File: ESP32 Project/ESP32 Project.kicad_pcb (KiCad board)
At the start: 4 copper layers, 49 x 38.3 mm, 27 parts, among them P1 USB_C_Plug_USB2.0, U1 ESP32-S3-WROOM-1-N8R2, U2 AMS1117, U3 BMP390, U4 INA219AxD, U5 LM75B, U6 SHTC3

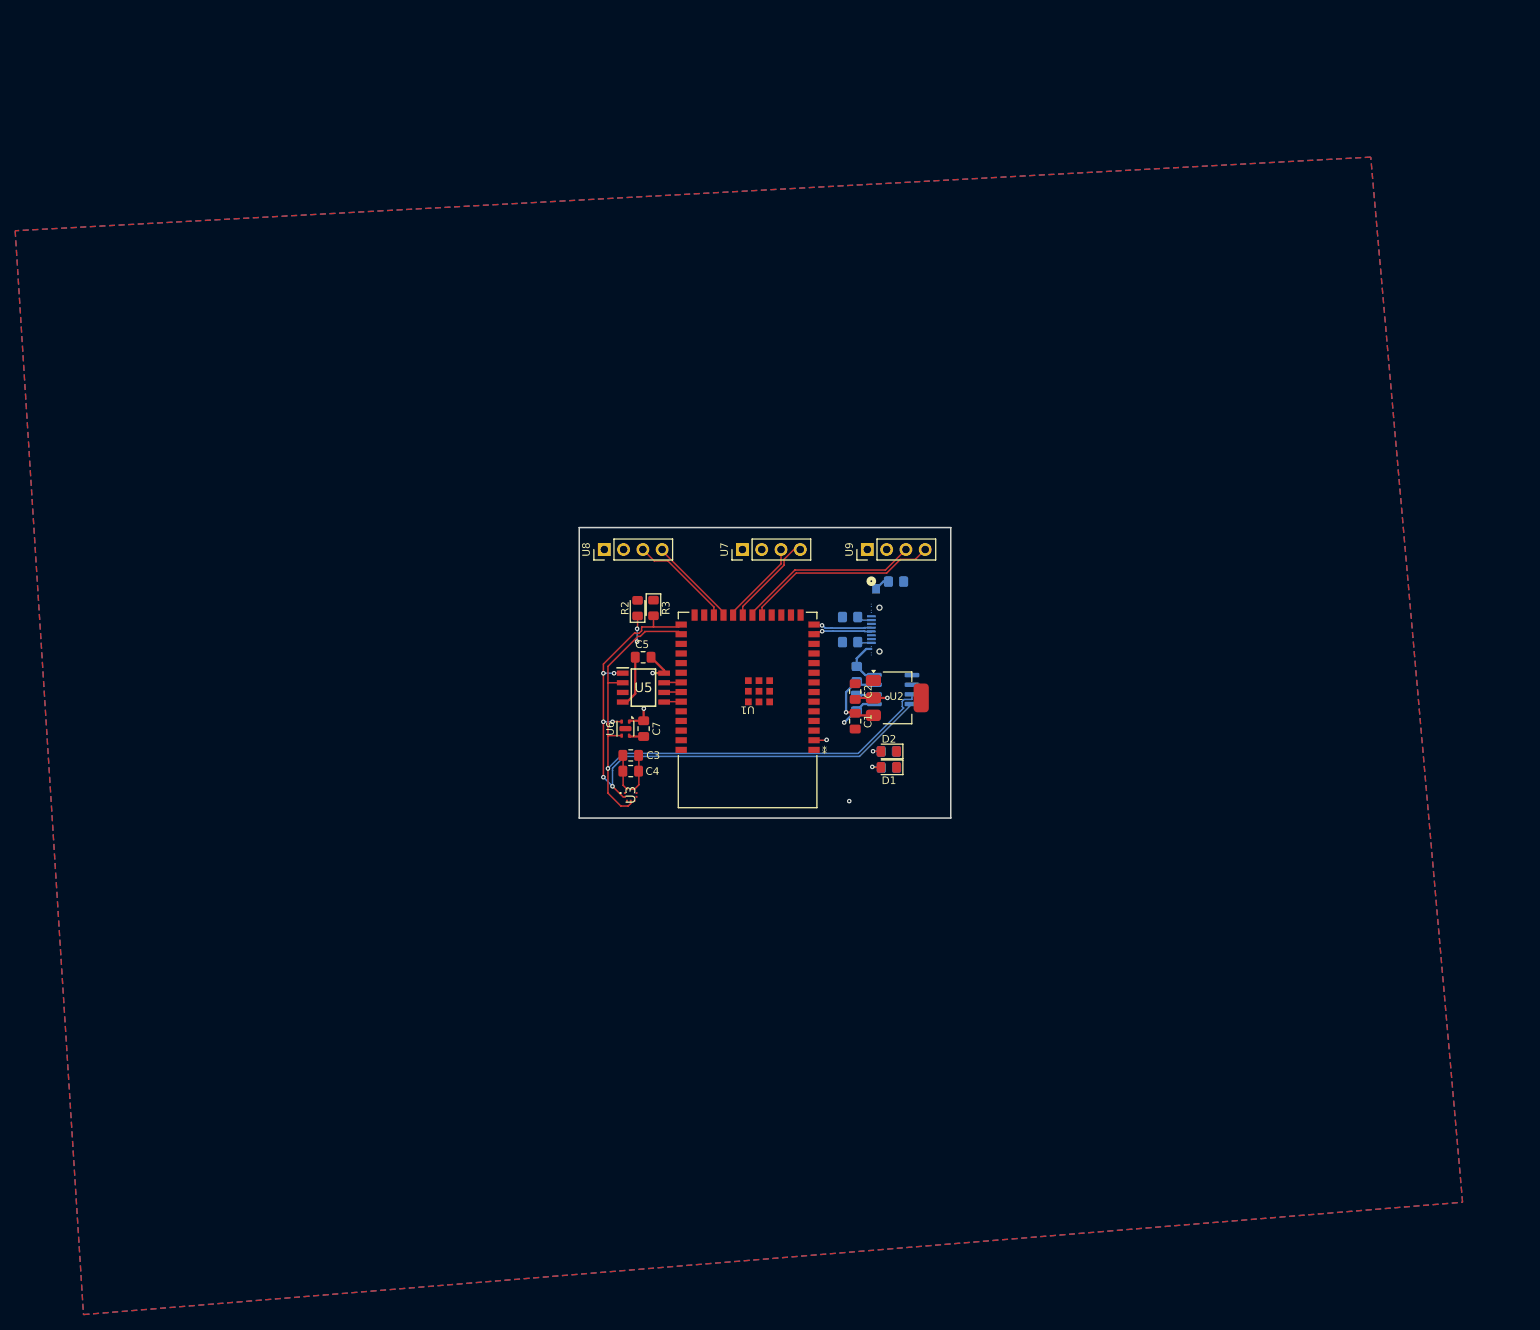
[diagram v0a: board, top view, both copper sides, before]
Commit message: newstuff
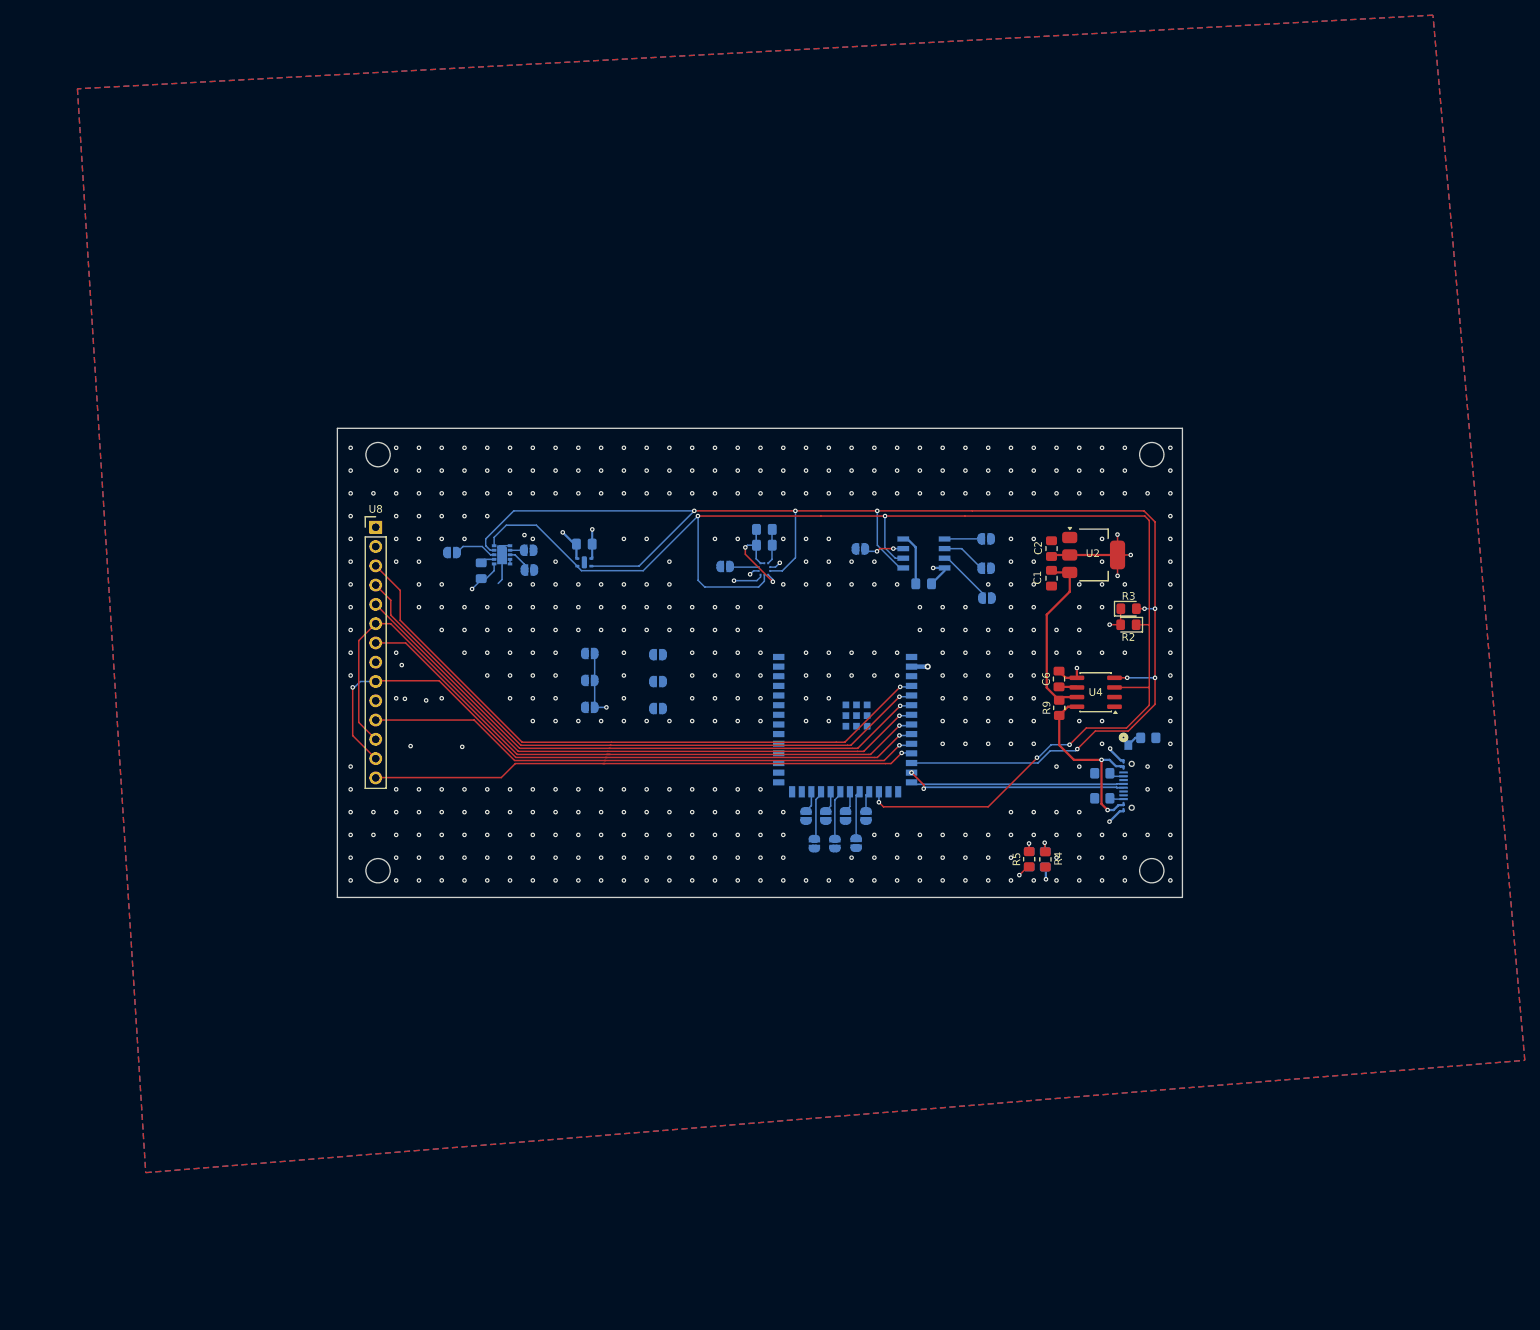
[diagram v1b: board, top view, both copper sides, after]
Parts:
- removed U9: ~, Connector_PinHeader_2.54mm:PinHeader_1x04_P2.54mm_Vertical
- added C8: 100nF, Capacitor_SMD:C_0805_2012Metric_Pad1.18x1.45mm_HandSolder, B.Cu at (107.4, 79.9)
- added JP1: SolderJumper_2_Open, Jumper:SolderJumper-2_P1.3mm_Open_RoundedPad1.0x1.5mm, B.Cu at (139.5, 79.3)
- added JP10: SolderJumper_2_Open, Jumper:SolderJumper-2_P1.3mm_Open_RoundedPad1.0x1.5mm, B.Cu at (156.8, 115.8)
- added JP11: SolderJumper_2_Open, Jumper:SolderJumper-2_P1.3mm_Open_RoundedPad1.0x1.5mm, B.Cu at (155.4, 112.2)
- added JP12: SolderJumper_2_Open, Jumper:SolderJumper-2_P1.3mm_Open_RoundedPad1.0x1.5mm, B.Cu at (154.0, 115.8)
- added JP13: SolderJumper_2_Open, Jumper:SolderJumper-2_P1.3mm_Open_RoundedPad1.0x1.5mm, B.Cu at (152.8, 112.2)
- added JP14: SolderJumper_2_Open, Jumper:SolderJumper-2_P1.3mm_Open_RoundedPad1.0x1.5mm, B.Cu at (151.3, 115.8)
- added JP15: SolderJumper_2_Open, Jumper:SolderJumper-2_P1.3mm_Open_RoundedPad1.0x1.5mm, B.Cu at (150.2, 112.2)
- added JP16: SolderJumper_2_Open, Jumper:SolderJumper-2_P1.3mm_Open_RoundedPad1.0x1.5mm, B.Cu at (130.7, 91.0)
- added JP17: SolderJumper_2_Open, Jumper:SolderJumper-2_P1.3mm_Open_RoundedPad1.0x1.5mm, B.Cu at (130.7, 94.5)
- added JP18: SolderJumper_2_Open, Jumper:SolderJumper-2_P1.3mm_Open_RoundedPad1.0x1.5mm, B.Cu at (130.7, 98.0)
- added JP19: SolderJumper_2_Open, Jumper:SolderJumper-2_P1.3mm_Open_RoundedPad1.0x1.5mm, B.Cu at (121.7, 90.8)
- added JP2: SolderJumper_2_Open, Jumper:SolderJumper-2_P1.3mm_Open_RoundedPad1.0x1.5mm, B.Cu at (174.0, 83.5)
- added JP20: SolderJumper_2_Open, Jumper:SolderJumper-2_P1.3mm_Open_RoundedPad1.0x1.5mm, B.Cu at (121.7, 94.3)
- added JP21: SolderJumper_2_Open, Jumper:SolderJumper-2_P1.3mm_Open_RoundedPad1.0x1.5mm, B.Cu at (121.7, 97.9)
- added JP3: SolderJumper_2_Open, Jumper:SolderJumper-2_P1.3mm_Open_RoundedPad1.0x1.5mm, B.Cu at (173.9, 79.6)
- added JP4: SolderJumper_2_Open, Jumper:SolderJumper-2_P1.3mm_Open_RoundedPad1.0x1.5mm, B.Cu at (173.9, 75.7)
- added JP5: SolderJumper_2_Open, Jumper:SolderJumper-2_P1.3mm_Open_RoundedPad1.0x1.5mm, B.Cu at (157.4, 77.0)
- added JP6: SolderJumper_2_Open, Jumper:SolderJumper-2_P1.3mm_Open_RoundedPad1.0x1.5mm, B.Cu at (113.7, 77.2)
- added JP7: SolderJumper_2_Open, Jumper:SolderJumper-2_P1.3mm_Open_RoundedPad1.0x1.5mm, B.Cu at (113.8, 79.8)
- added JP8: SolderJumper_2_Open, Jumper:SolderJumper-2_P1.3mm_Open_RoundedPad1.0x1.5mm, B.Cu at (103.5, 77.5)
- added JP9: SolderJumper_2_Open, Jumper:SolderJumper-2_P1.3mm_Open_RoundedPad1.0x1.5mm, B.Cu at (158.1, 112.2)
- C3, C4, C5, C7, D1, D2, U1, U3, U5, U6: moved to B.Cu
- C6, R4, R5, R9, U4: moved to F.Cu
- U7: value ~ -> CCS811; footprint Connector_PinHeader_2.54mm:PinHeader_1x04_P2.54mm_Vertical -> Package_LGA:AMS_LGA-10-1EP_2.7x4mm_P0.6mm; moved to B.Cu
- U8: footprint Connector_PinHeader_2.54mm:PinHeader_1x04_P2.54mm_Vertical -> Connector_PinHeader_2.54mm:PinHeader_1x14_P2.54mm_Vertical
- moved R2 64.7 mm to (192.7, 87.0), turned to 180 degrees
- moved R3 62.6 mm to (192.7, 84.9), turned to 0 degrees
- moved U5 41.0 mm to (165.7, 77.6)
- moved R7 39.1 mm to (189.2, 109.9)
- moved P1 39.1 mm to (195.7, 108.2)
- moved R1 39.1 mm to (195.3, 101.9)
- moved R6 39.1 mm to (189.2, 106.6)
- moved C5 38.2 mm to (165.7, 81.6)
- moved C3 34.6 mm to (144.7, 74.5), turned to 180 degrees
- moved C4 34.6 mm to (144.7, 76.5), turned to 180 degrees
- moved U3 34.6 mm to (144.7, 79.7)
- moved C1 32.0 mm to (182.5, 80.9)
- moved U2 32.0 mm to (188.1, 77.8)
- moved C2 32.0 mm to (182.5, 77.0)
- moved U7 31.7 mm to (110.2, 77.8), turned to 180 degrees
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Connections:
- U1 pad 10: unconnected-(U1-IO17-Pad10) -> Net-(U1-IO17)
- U1 pad 11: unconnected-(U1-IO18-Pad11) -> Net-(U1-IO18)
- U1 pad 12: unconnected-(U1-IO8-Pad12) -> SDA
- U1 pad 17: unconnected-(U1-IO9-Pad17) -> SCL
- U1 pad 18: unconnected-(U1-IO10-Pad18) -> Net-(JP9-A)
- U1 pad 19: SCA_OLED3 -> Net-(JP10-A)
- U1 pad 20: SCL_OLED3 -> Net-(JP11-A)
- U1 pad 21: SCA_OLED2 -> Net-(JP12-A)
- U1 pad 22: SCL_OLED2 -> Net-(JP13-A)
- U1 pad 23: SCA_OLED1 -> Net-(JP14-A)
- U1 pad 24: SCL_OLED1 -> Net-(JP15-A)
- U1 pad 27: SDA -> unconnected-(U1-IO0-Pad27)
- U1 pad 28: SCL -> unconnected-(U1-IO35-Pad28)
- U1 pad 4: unconnected-(U1-IO4-Pad4) -> Net-(U1-IO4)
- U1 pad 5: unconnected-(U1-IO5-Pad5) -> Net-(U1-IO5)
- U1 pad 6: unconnected-(U1-IO6-Pad6) -> Net-(U1-IO6)
- U1 pad 7: unconnected-(U1-IO7-Pad7) -> Net-(U1-IO7)
- U1 pad 8: unconnected-(U1-IO15-Pad8) -> Net-(U1-IO15)
- U1 pad 9: unconnected-(U1-IO16-Pad9) -> Net-(U1-IO16)
- U3 pad 7: unconnected-(U3-INT-Pad7) -> Net-(JP1-A)
- U5 pad 3: unconnected-(U5-O.S.-Pad3) -> Net-(JP5-A)
- U5 pad 5: A0_TEMP -> Net-(JP4-A)
- U5 pad 6: A1_TEMP -> Net-(JP3-A)
- U5 pad 7: A2_TEMP -> Net-(JP2-A)
- U7 pad 2: +3.3V -> Net-(JP6-A)
- U7 pad 3: SCL_OLED2 -> Net-(JP7-A)
- U7 pad 4: SCA_OLED2 -> Net-(U7-PWM)
- U8 pad 1: GND -> +3.3V
- U8 pad 2: +3.3V -> GND
- U8 pad 3: SCL_OLED1 -> Net-(U1-IO4)
- U8 pad 4: SCA_OLED1 -> Net-(U1-IO5)
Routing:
- net SDA: track 83.3 -> 195.7 mm, vias 6 -> 8
- net SCL: track 85.1 -> 193.3 mm, vias 3 -> 5
- net Net-(U1-IO7): track 0.00 -> 96.7 mm, vias 0 -> 1
- net Net-(U1-IO16): track 0.00 -> 90.3 mm, vias 0 -> 2
- net Net-(U1-IO4): track 0.00 -> 85.6 mm, vias 0 -> 1
- net Net-(U1-IO5): track 0.00 -> 83.3 mm, vias 0 -> 1
- net Net-(U1-IO6): track 0.00 -> 81.0 mm, vias 0 -> 1
- net Net-(U1-IO15): track 0.00 -> 78.8 mm, vias 0 -> 1
- net Net-(U1-IO17): track 0.00 -> 73.9 mm, vias 0 -> 1
- net Net-(U1-IO18): track 0.00 -> 72.3 mm, vias 0 -> 1
- net +3.3V: track 18.9 -> 51.6 mm, vias 5 -> 13
- net SCA_OLED3: track 25.7 -> 0.00 mm
- net SCL_OLED3: track 24.0 -> 0.00 mm
- net D-: track 7.75 -> 29.2 mm, vias 1 -> 2
- net GND: track 10.7 -> 31.1 mm, vias 1 -> 473
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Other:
- board size 49 x 38.3 mm -> 111.3 x 61.8 mm
- board text added: "SMART HOME MONITOR"
- board text added: "v1.1"
- board text added: "{ "ViaStitching": "0.2", "stitch_zone_0": { "HSpacing": "1", "VSpacing": "1", "HOffset": "0", "VOffset": "0", "Clearance": "0.3", "Randomize": false } }"
- board text added: "{ "ViaStitching": "0.2", "stitch_zone_0": { "HSpacing": "1", "VSpacing": "1", "HOffset": "0", "VOffset": "0", "Clearance": "5", "Randomize": false } }"
- board text added: "{ "ViaStitching": "0.2", "stitch_zone_0": { "HSpacing": "2.5", "VSpacing": "2.5", "HOffset": "0", "VOffset": "0", "Clearance": "0.4", "Randomize": false } }"
- board text added: "{ "ViaStitching": "0.2", "stitch_zone_0": { "HSpacing": "2.5", "VSpacing": "2.5", "HOffset": "0", "VOffset": "0", "Clearance": "0.5", "Randomize": false } }"
- board text added: "{ "ViaStitching": "0.2", "stitch_zone_0": { "HSpacing": "3", "VSpacing": "3", "HOffset": "0", "VOffset": "0", "Clearance": "0.4", "Randomize": false } }"
